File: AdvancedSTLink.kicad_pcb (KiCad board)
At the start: 4 copper layers, 49.9 x 23.1 mm, 56 parts, among them J1 USB_C_Receptacle, J2 Conn_02x03_Odd_Even, J3 Conn_01x06, J4 Conn_02x03_Odd_Even, Q1 S8050, SW1 SW_SPDT, U1 STM32F205RETx, U2 XC6206P332MR, U3 USBLC6-2P6, U4 GM9038, U5 USBLC6-2P6, U6 USBLC6-2P6, Y1 X322512MSB4SI

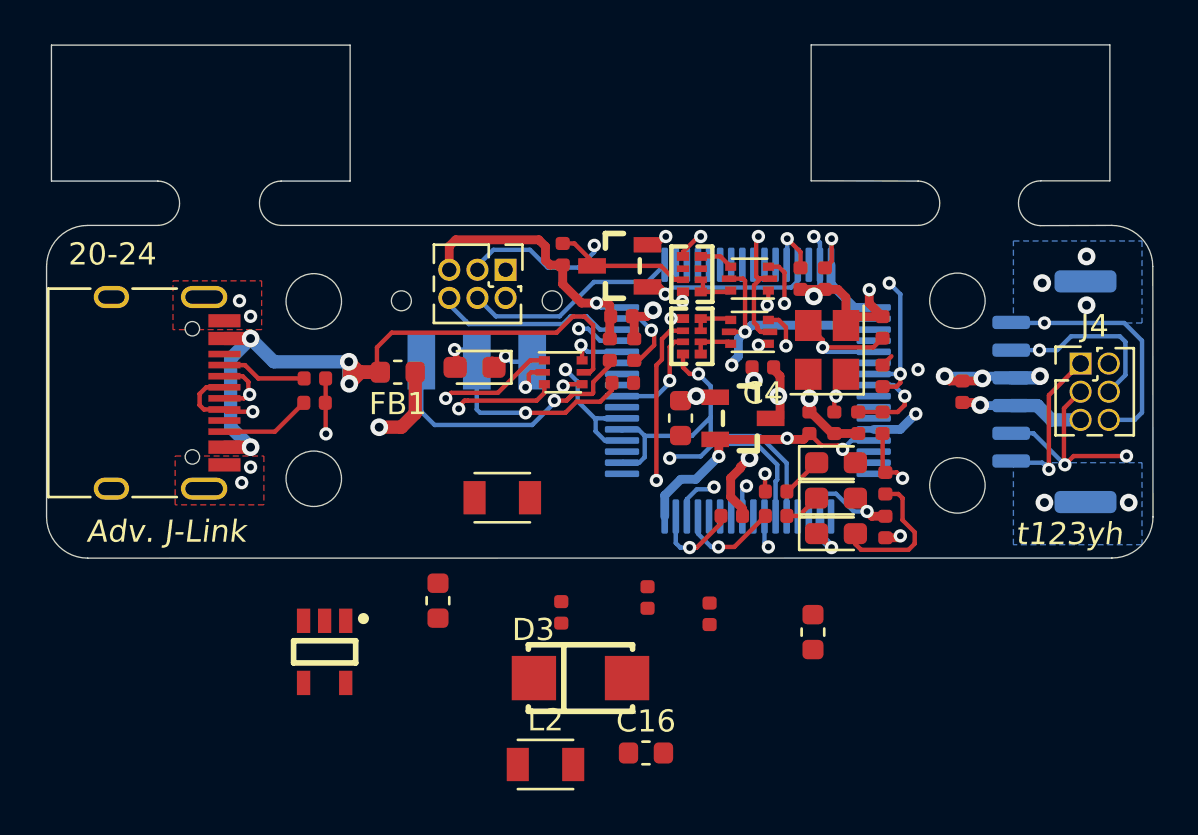
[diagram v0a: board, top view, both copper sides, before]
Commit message: Layout.
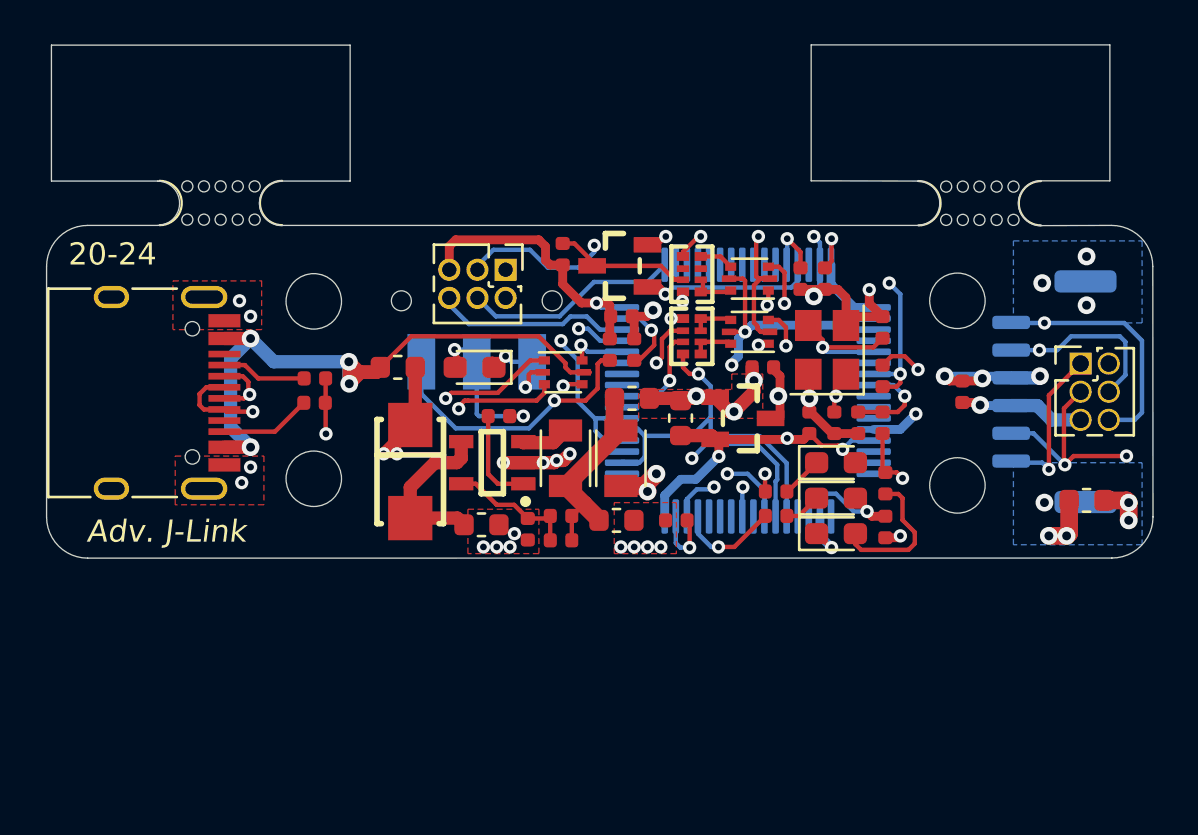
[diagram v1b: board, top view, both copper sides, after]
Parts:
- added C17: 10uF, Capacitor_SMD:C_0603_1608Metric, F.Cu at (188.6, 104.8)
- added H5: MouseBite, mouse_bite:mouse-bite-3mm-slot, F.Cu at (170.1, 96.0)
- added H6: MouseBite, mouse_bite:mouse-bite-3mm-slot, F.Cu at (204.3, 96.0)
- C12: value 22uF -> 10uF
- moved C16 22.9 mm to (209.1, 109.4)
- moved L2 14.2 mm to (188.1, 107.5), turned to 270 degrees
- moved D3 12.1 mm to (178.6, 108.1), turned to 270 degrees
- moved U4 11.4 mm to (182.3, 107.7), turned to 0 degrees
- moved C12 10.2 mm to (187.9, 110.3), turned to 0 degrees
- moved R15 9.04 mm to (183.9, 110.7), turned to 90 degrees
- moved R1 5.78 mm to (182.6, 105.6), turned to 0 degrees
- moved R14 4.68 mm to (185.4, 111.2), turned to 0 degrees
- moved C7 4.35 mm to (185.4, 110.1), turned to 180 degrees
- moved C6 3.95 mm to (181.8, 110.5), turned to 0 degrees
- moved L1 3.36 mm to (185.6, 107.5), turned to 270 degrees
- moved C13 2.51 mm to (190.6, 110.3), turned to 0 degrees
- moved FB1 0.22 mm to (178.0, 103.4)
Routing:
- net GND: track 47.8 -> 57.6 mm, vias 29 -> 42
- net Net-(C12-Pad1): track 0.00 -> 9.14 mm
- net Net-(C6-Pad1): track 0.00 -> 7.53 mm
- net Net-(C7-Pad2): track 0.00 -> 5.81 mm
- net V_OUT_3.3: track 38.1 -> 42.9 mm, vias 2 -> 6
- net Net-(R1-Pad1): track 0.00 -> 4.38 mm
- net Net-(D6-Pad2): track 12.6 -> 8.67 mm
- net TMS2: track 16.4 -> 13.0 mm
- net Net-(FB1-Pad2): track 31.9 -> 28.6 mm
- net VBUS: track 31.6 -> 34.2 mm, vias 2 -> 3
- net Net-(L1-Pad1): track 0.00 -> 2.53 mm
- net +3V3: track 68.6 -> 69.8 mm
- net Net-(C13-Pad2): track 4.29 -> 3.36 mm
- net TMS1: track 15.4 -> 14.7 mm
- net Net-(R9-Pad2): track 13.1 -> 12.6 mm
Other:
- board text removed: "t123yh"

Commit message: Layout optimizations.
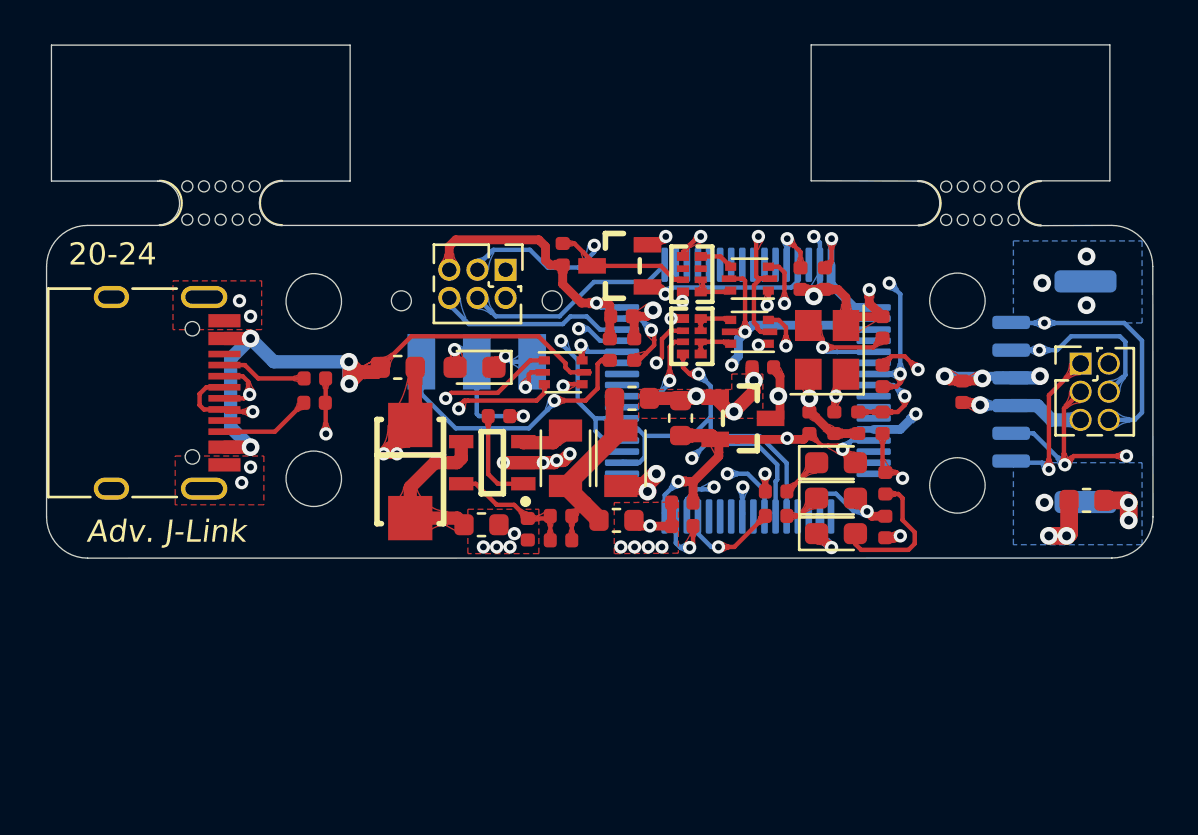
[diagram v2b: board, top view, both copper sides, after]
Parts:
- added C18: 100nF, Capacitor_SMD:C_0402_1005Metric, F.Cu at (190.9, 109.5)
- D5: value LED_Blue -> LED_Green
- R16: value 1.5k -> 2.2k
- moved C13 0.37 mm to (190.9, 110.6)
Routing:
- net GND: track 57.6 -> 60.5 mm, vias 42 -> 43
- net +3V3: track 69.8 -> 70.8 mm

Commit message: Fixes.
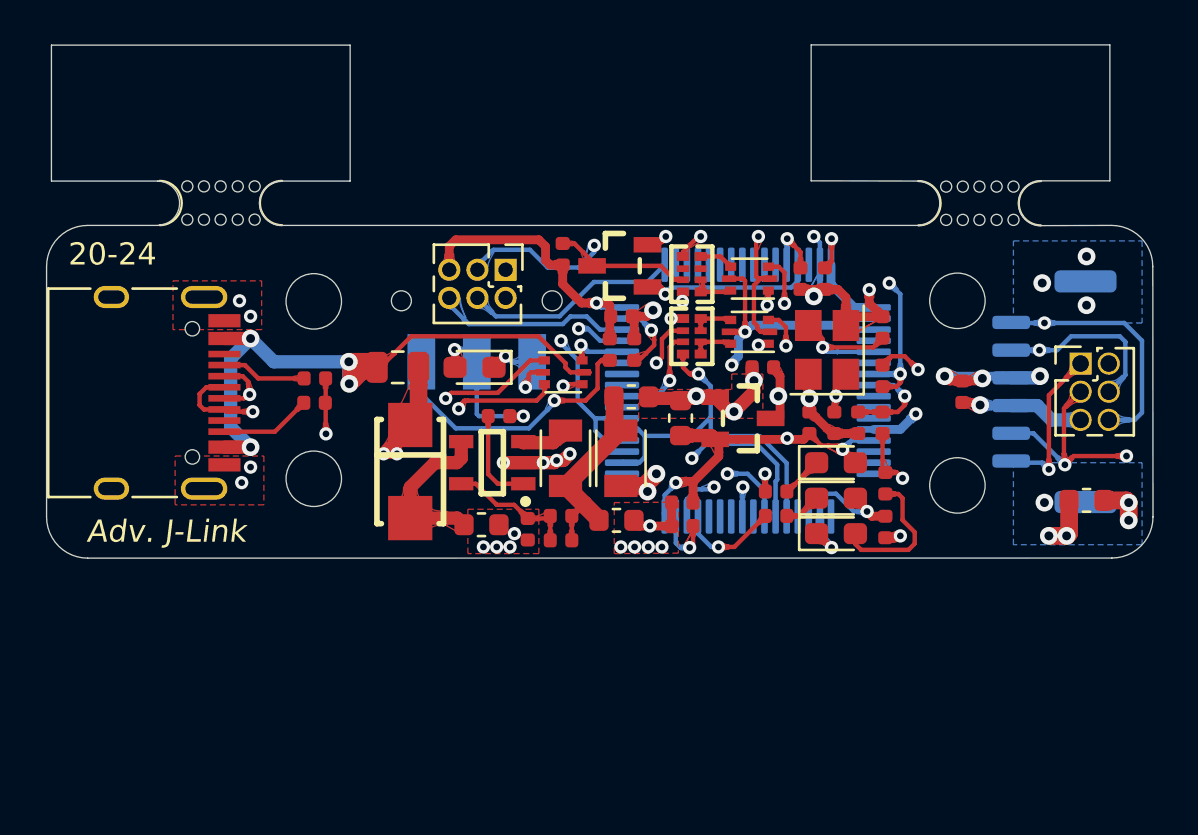
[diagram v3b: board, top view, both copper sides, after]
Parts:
- FB1: footprint Inductor_SMD:L_0603_1608Metric -> Inductor_SMD:L_0805_2012Metric
- moved C17 0.08 mm to (188.6, 104.7)
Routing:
- net VBUS: track 34.2 -> 35.1 mm
